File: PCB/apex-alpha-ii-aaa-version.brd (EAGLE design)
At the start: 13.1 x 74.7 mm, 36 parts, among them IC1 CC430F5135, IC2 TPS61200, Y1 26MHz

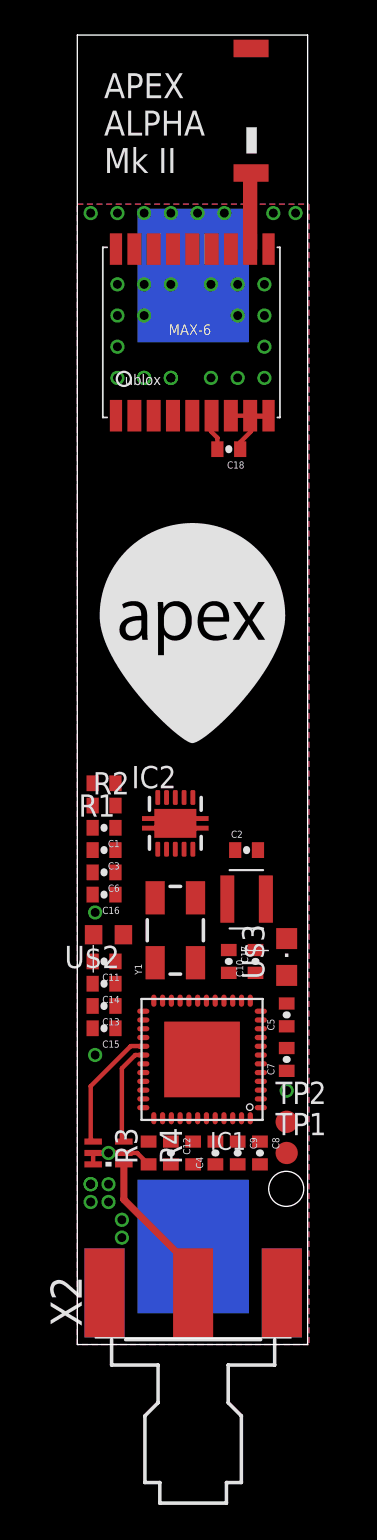
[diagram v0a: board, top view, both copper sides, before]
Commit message: Nearly finished routing... committing before I lose it all.
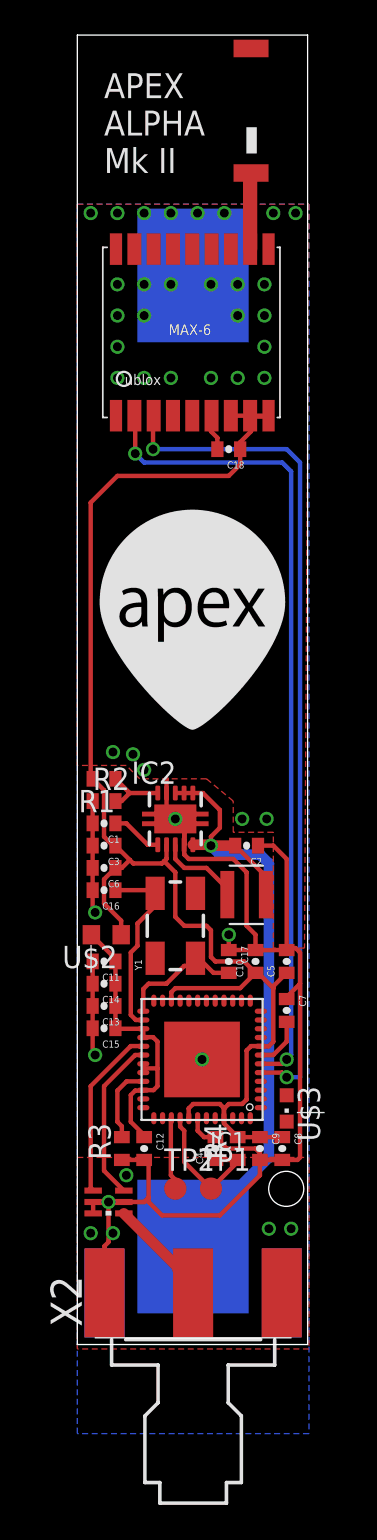
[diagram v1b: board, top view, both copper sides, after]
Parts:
- U$3: device apex:CHIPLED_0805 -> apex:CHIPLED_0603
- moved U$3 8.64 mm to (11.9, 13.5), turned to 180 degrees
- moved TP2 7.41 mm to (5.59, 8.89)
- moved TP1 4.77 mm to (7.62, 8.89)
- moved C5 3.05 mm to (11.9, 21.8)
- moved C7 2.79 mm to (11.9, 19.1), turned to 270 degrees
- moved F1 2.79 mm to (1.78, 8.13)
- moved R4 2.55 mm to (9.14, 11.2)
- moved R3 1.55 mm to (2.54, 11.2)
- moved C12 1.55 mm to (3.81, 11.2)
- moved C8 1.30 mm to (11.7, 11.2)
- moved C9 1.30 mm to (10.4, 11.2)
- moved U$4 0.76 mm to (1.27, 35.1)
- moved R1 0.25 mm to (1.52, 32.3)
- moved C1 0.25 mm to (1.52, 29.7)
- moved C16 0.25 mm to (1.52, 25.9)
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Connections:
- removed net PP: IC2.PP, IC2.PP@1, IC2.PP@2
- net GND: now also IC2.PP, IC2.PP@1, IC2.PP@2
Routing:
- net GND: track 9.84 -> 88.4 mm, vias 39 -> 42
- net VCC: track 5.36 -> 81.1 mm
- net GPSRX: track 0.00 -> 48.0 mm, vias 0 -> 2
- net GPSTX: track 0.00 -> 46.7 mm, vias 0 -> 2
- net N$1: track 0.00 -> 38.5 mm, vias 0 -> 1
- net VEE: track 0.00 -> 17.5 mm
- net N$14: track 0.00 -> 10.7 mm
- net N$11: track 0.00 -> 8.28 mm
- net N$13: track 0.00 -> 7.21 mm
- net N$3: track 0.00 -> 4.81 mm
- net N$9: track 0.00 -> 4.45 mm
- net N$12: track 0.00 -> 4.13 mm
- net N$4: track 0.00 -> 3.75 mm
- net N$2: track 5.76 -> 9.40 mm
- net N$6: track 7.19 -> 10.2 mm
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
